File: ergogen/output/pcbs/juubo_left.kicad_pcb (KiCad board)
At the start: 2 copper layers, 145.5 x 125.5 mm, 47 parts

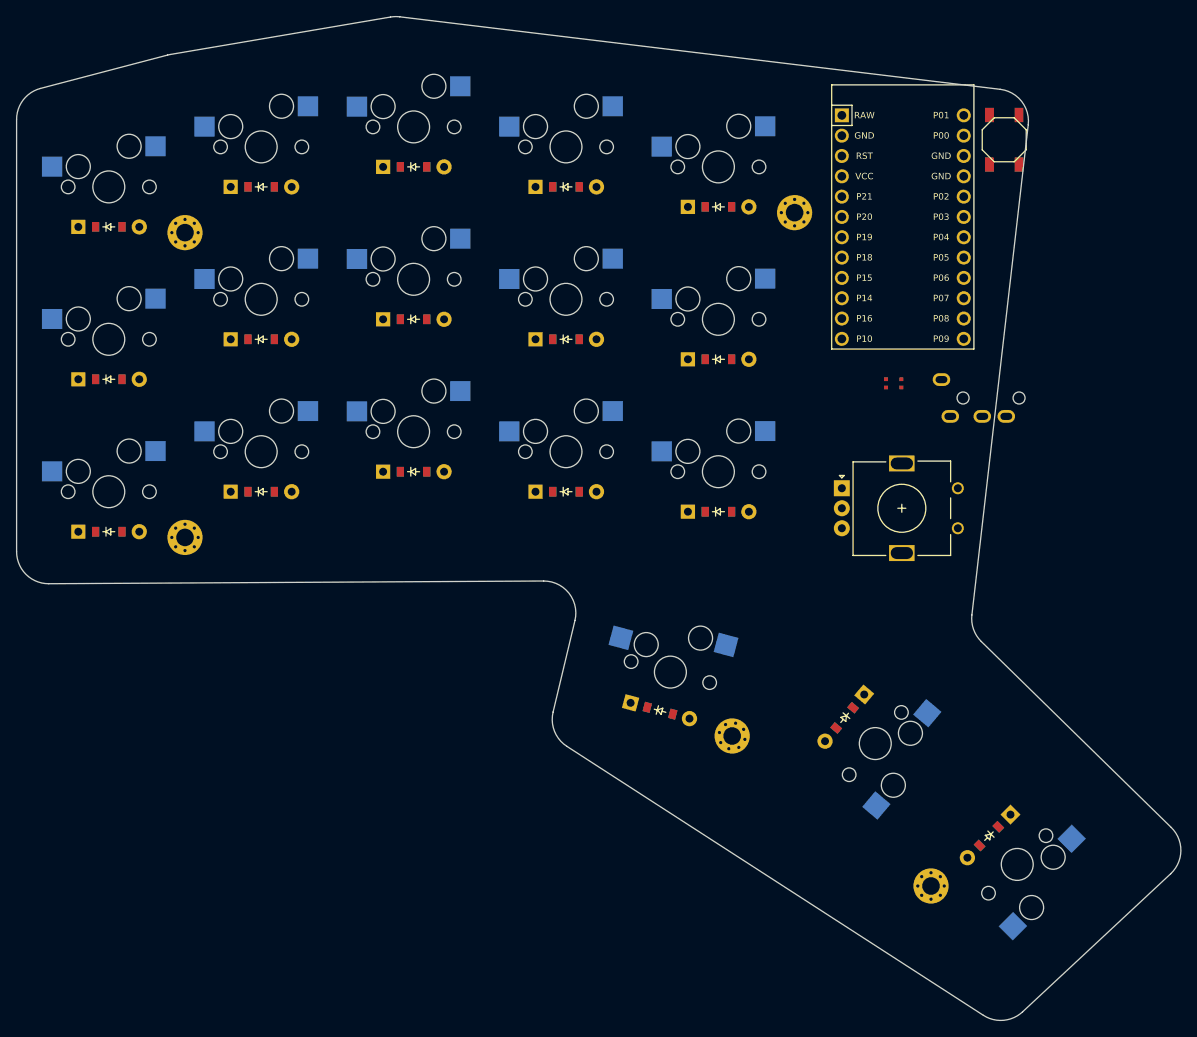
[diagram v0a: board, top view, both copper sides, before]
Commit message: Diode pads routed
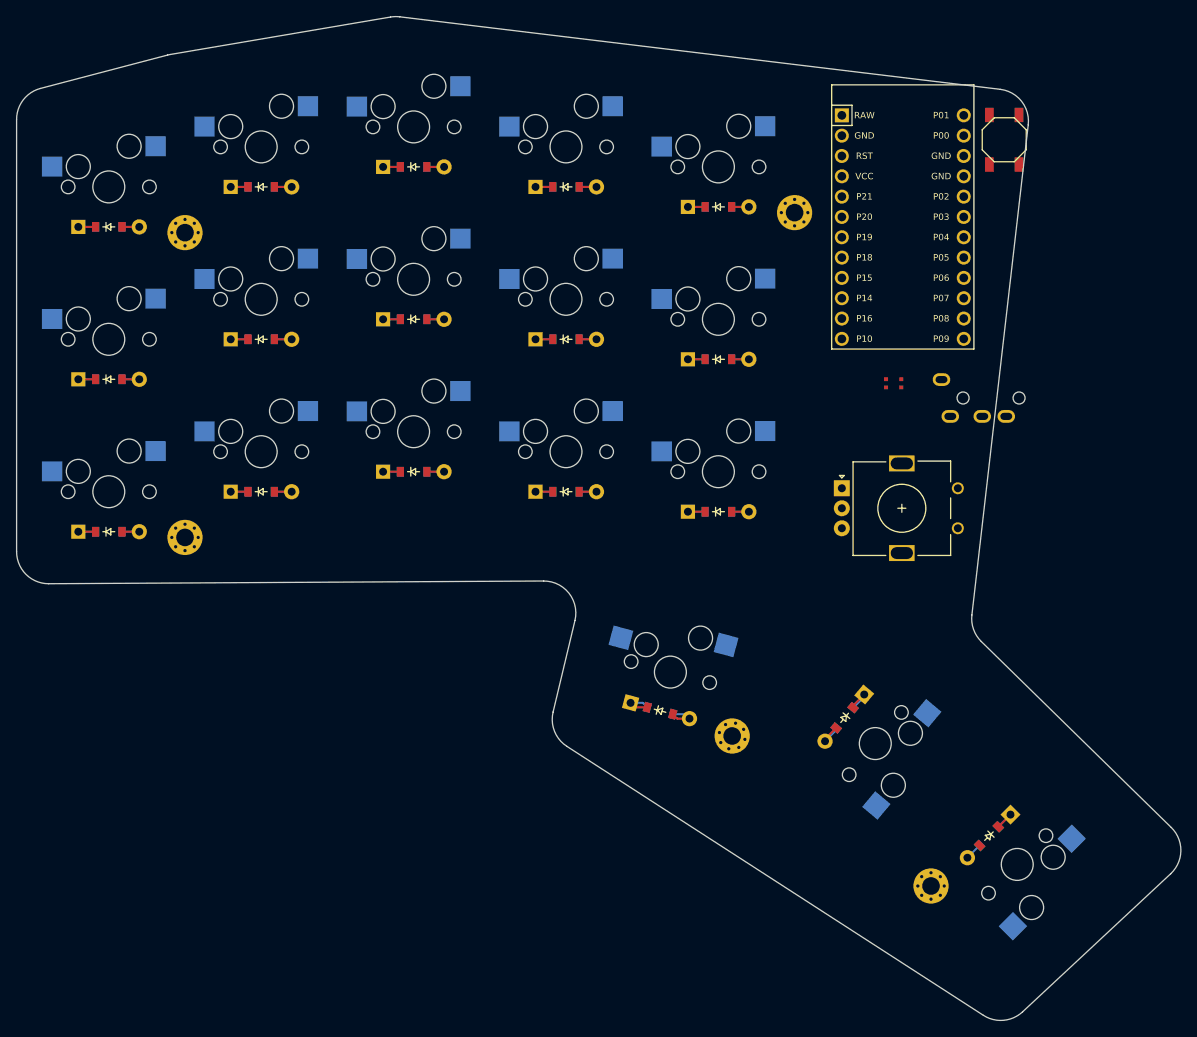
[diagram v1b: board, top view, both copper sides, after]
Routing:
- net P16: track 0.00 -> 21.6 mm
- net P15: track 0.00 -> 21.6 mm
- net P14: track 0.00 -> 21.6 mm
- net P10: track 0.00 -> 13.4 mm
- net layer_cluster: track 0.00 -> 4.64 mm
- net inner_home: track 0.00 -> 4.53 mm
- net space_cluster: track 0.00 -> 4.46 mm
- net ring_top: track 0.00 -> 4.32 mm
- net ring_home: track 0.00 -> 4.32 mm
- net ring_bottom: track 0.00 -> 4.32 mm
- net pinky_top: track 0.00 -> 4.32 mm
- net pinky_home: track 0.00 -> 4.32 mm
- net pinky_bottom: track 0.00 -> 4.32 mm
- net middle_top: track 0.00 -> 4.32 mm
- net middle_home: track 0.00 -> 4.32 mm
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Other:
- net class Default removed
